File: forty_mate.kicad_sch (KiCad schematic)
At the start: 94 parts, among them SW1 SW_Push, SW10 SW_Push, SW11 SW_Push, SW12 SW_Push, SW13 SW_Push, SW14 SW_Push, SW15 SW_Push, SW16 SW_Push, SW17 SW_Push, SW18 SW_Push, SW19 SW_Push, SW2 SW_Push, SW20 SW_Push, SW21 SW_Push, SW22 SW_Push, SW23 SW_Push, SW24 SW_Push, SW25 SW_Push, SW26 SW_Push, SW27 SW_Push, SW28 SW_Push, SW29 SW_Push, SW3 SW_Push, SW30 SW_Push, SW31 SW_Push, SW32 SW_Push, SW33 SW_Push, SW34 SW_Push, SW35 SW_Push, SW36 SW_Push, SW37 SW_Push, SW38 SW_Push, SW39 SW_Push, SW4 SW_Push, SW40 SW_Push, SW41 SW_Push, SW42 SW_Push, SW43 SW_Push, SW44 SW_SPDT, SW5 SW_Push, SW6 SW_Push, SW7 SW_Push, SW8 SW_Push, SW9 SW_Push, U1 Micon_BLEMicroPro

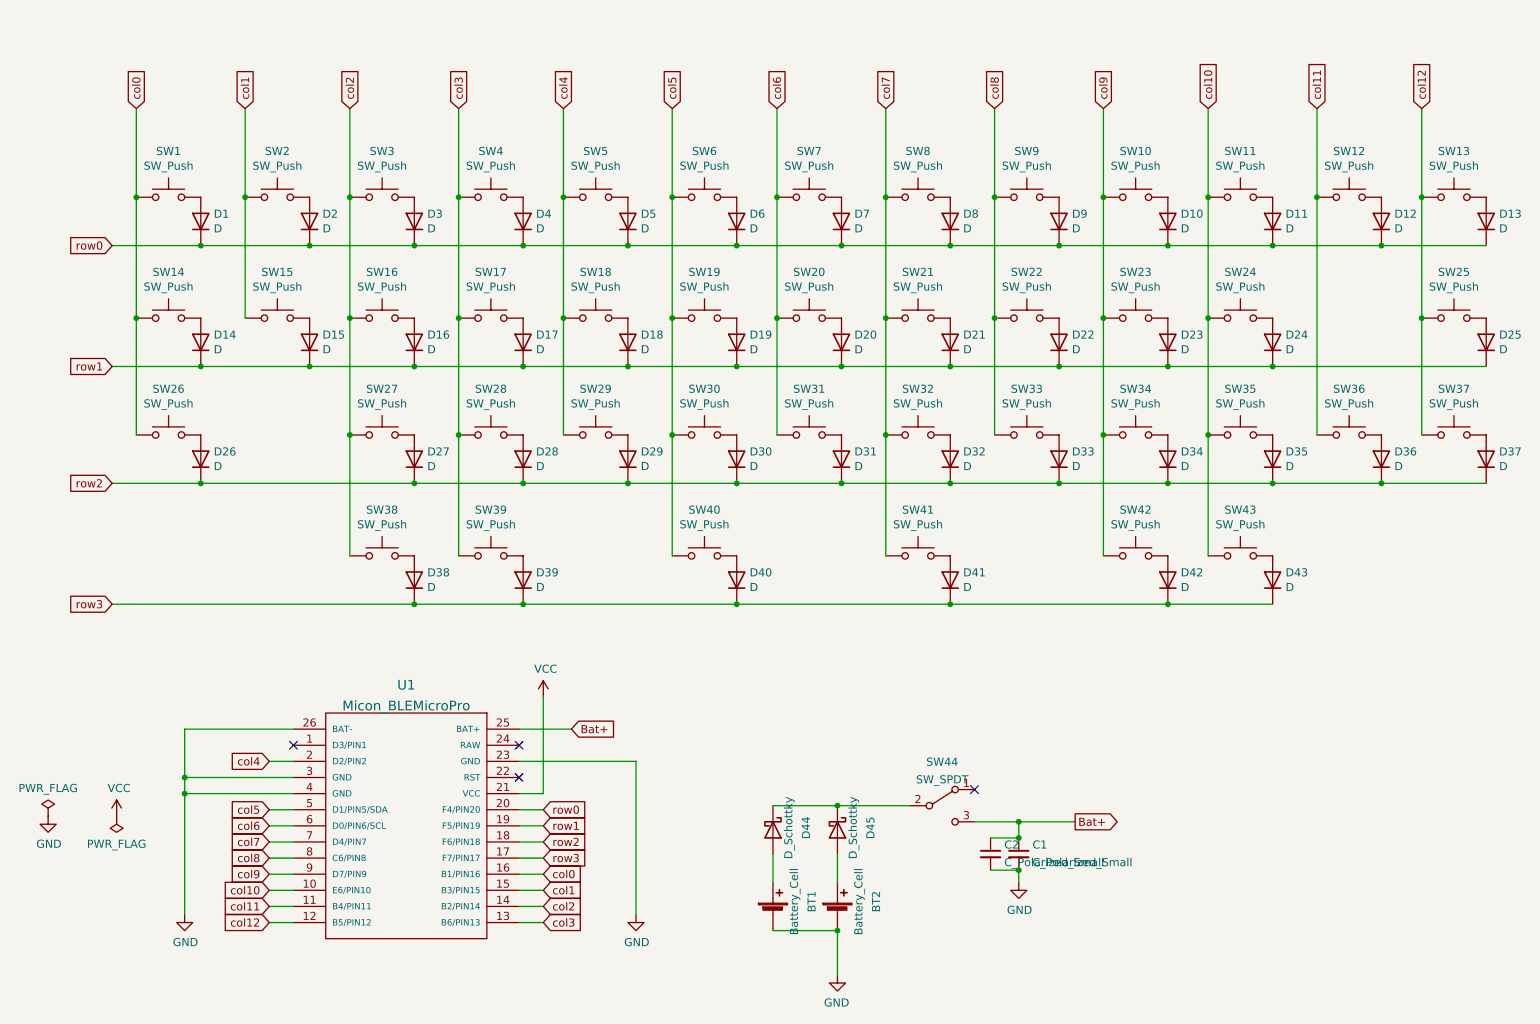
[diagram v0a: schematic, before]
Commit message: kari kansei
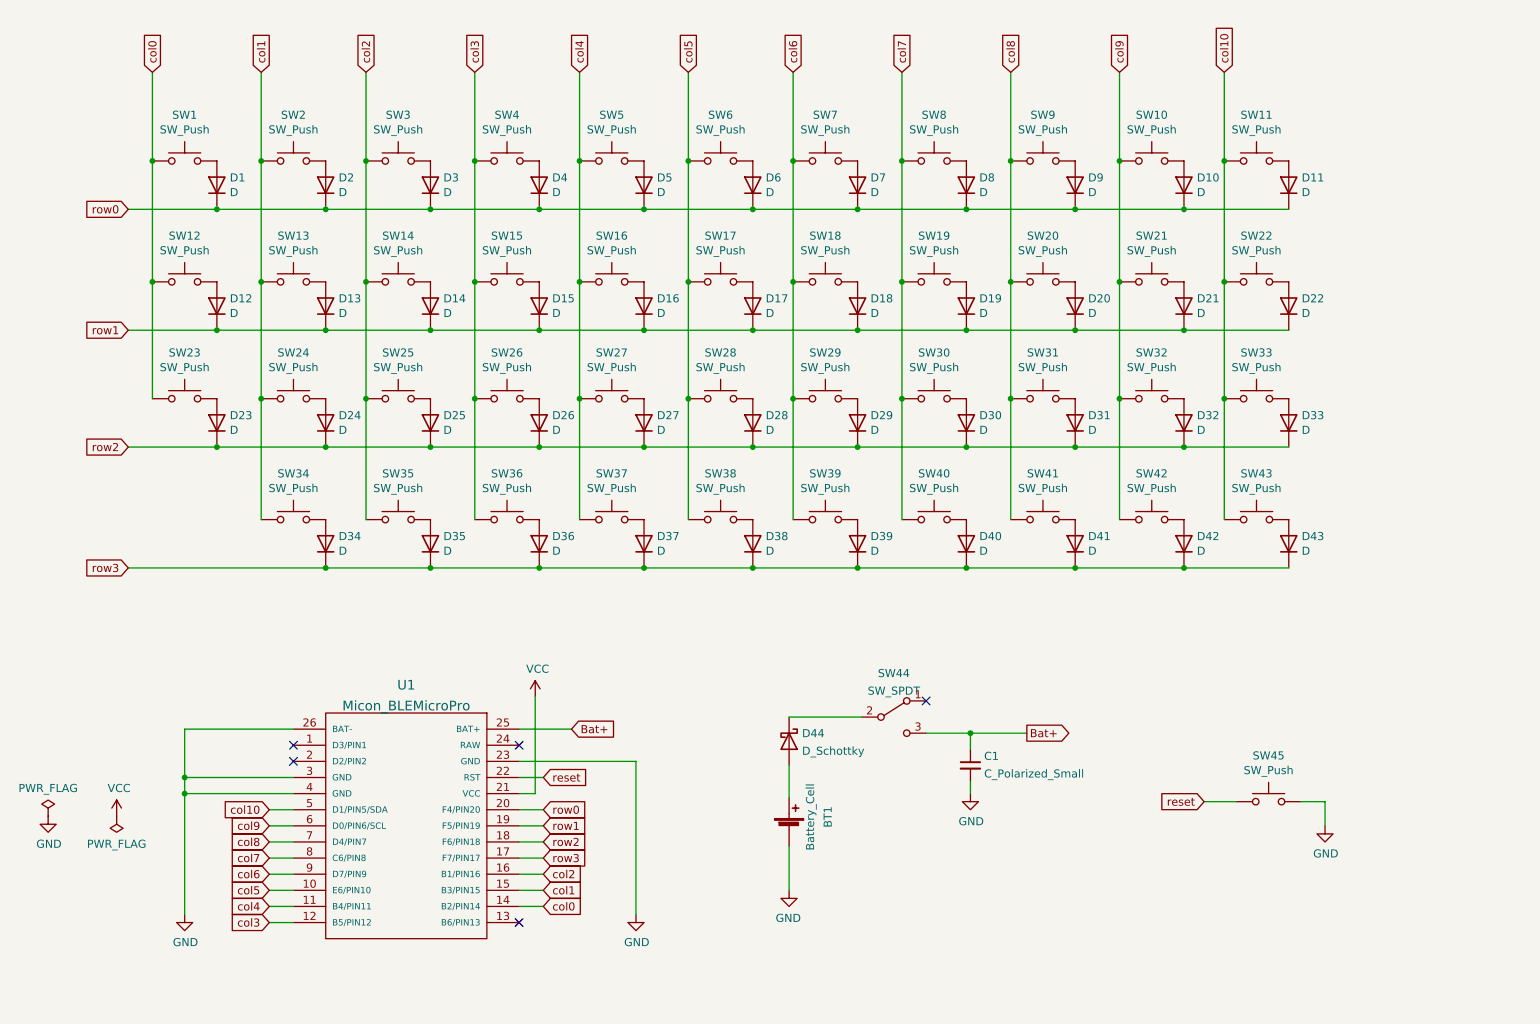
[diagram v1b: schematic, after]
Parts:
- removed BT1: Battery_Cell, kbd_Parts:Battery_ali_CR1632, symbol Device:Battery_Cell
- removed C2: C_Polarized_Small, kbd_Parts:Capacitor_1206, symbol Device:C_Small
- removed D12, D13, D25: D, kbd_Parts:Diode_TH_SMD, symbol Device:D
- removed D45: D_Schottky, kbd_Parts:Diode_TH_SMD, symbol Device:D_Schottky
- removed SW12, SW13, SW25: SW_Push, kbd_SW:CherryMX_Hotswap_1u, symbol Switch:SW_Push
- added D34, D39, D41: D, kbd_Parts:Diode_SMD, symbol Device:D
- added SW34, SW39, SW41: SW_Push, kbd_SW:CherryMX_Hotswap_1u, symbol Switch:SW_Push
- added SW45: SW_Push, kbd_Parts:ResetSW, symbol Switch:SW_Push
- D1, D10, D11, D2, D3, D37, D4, D42, D43, D5, D6, D7, D8, D9: footprint kbd_Parts:Diode_TH_SMD -> kbd_Parts:Diode_SMD
- D12: renamed from D14; footprint kbd_Parts:Diode_TH_SMD -> kbd_Parts:Diode_SMD
- D13: renamed from D15; footprint kbd_Parts:Diode_TH_SMD -> kbd_Parts:Diode_SMD
- D14: renamed from D16; footprint kbd_Parts:Diode_TH_SMD -> kbd_Parts:Diode_SMD
- D15: renamed from D17; footprint kbd_Parts:Diode_TH_SMD -> kbd_Parts:Diode_SMD
- D16: renamed from D18; footprint kbd_Parts:Diode_TH_SMD -> kbd_Parts:Diode_SMD
- D17: renamed from D19; footprint kbd_Parts:Diode_TH_SMD -> kbd_Parts:Diode_SMD
- D18: renamed from D20; footprint kbd_Parts:Diode_TH_SMD -> kbd_Parts:Diode_SMD
- D19: renamed from D21; footprint kbd_Parts:Diode_TH_SMD -> kbd_Parts:Diode_SMD
- D20: renamed from D22; footprint kbd_Parts:Diode_TH_SMD -> kbd_Parts:Diode_SMD
- D21: renamed from D23; footprint kbd_Parts:Diode_TH_SMD -> kbd_Parts:Diode_SMD
- D22: renamed from D24; footprint kbd_Parts:Diode_TH_SMD -> kbd_Parts:Diode_SMD
- D23: renamed from D26; footprint kbd_Parts:Diode_TH_SMD -> kbd_Parts:Diode_SMD
- D24: renamed from D36; footprint kbd_Parts:Diode_TH_SMD -> kbd_Parts:Diode_SMD
- D25: renamed from D27; footprint kbd_Parts:Diode_TH_SMD -> kbd_Parts:Diode_SMD
- D26: renamed from D28; footprint kbd_Parts:Diode_TH_SMD -> kbd_Parts:Diode_SMD
- D27: renamed from D29; footprint kbd_Parts:Diode_TH_SMD -> kbd_Parts:Diode_SMD
- D28: renamed from D30; footprint kbd_Parts:Diode_TH_SMD -> kbd_Parts:Diode_SMD
- D29: renamed from D31; footprint kbd_Parts:Diode_TH_SMD -> kbd_Parts:Diode_SMD
- D30: renamed from D32; footprint kbd_Parts:Diode_TH_SMD -> kbd_Parts:Diode_SMD
- D31: renamed from D33; footprint kbd_Parts:Diode_TH_SMD -> kbd_Parts:Diode_SMD
- D32: renamed from D34; footprint kbd_Parts:Diode_TH_SMD -> kbd_Parts:Diode_SMD
- D33: renamed from D35; footprint kbd_Parts:Diode_TH_SMD -> kbd_Parts:Diode_SMD
- D35: renamed from D38; footprint kbd_Parts:Diode_TH_SMD -> kbd_Parts:Diode_SMD
- D36: renamed from D39; footprint kbd_Parts:Diode_TH_SMD -> kbd_Parts:Diode_SMD
- D38: renamed from D40; footprint kbd_Parts:Diode_TH_SMD -> kbd_Parts:Diode_SMD
- D40: renamed from D41; footprint kbd_Parts:Diode_TH_SMD -> kbd_Parts:Diode_SMD
- D44: footprint kbd_Parts:Diode_TH_SMD -> forty_mate:Diode_SMD_S-FLAT
- SW12: renamed from SW14; footprint kbd_SW:CherryMX_Hotswap_1u -> kbd_SW:CherryMX_Hotswap_1.25u
- SW23: renamed from SW26; footprint kbd_SW:CherryMX_Hotswap_1u -> kbd_SW:CherryMX_Hotswap_1.75u
- SW35: renamed from SW38; footprint kbd_SW:CherryMX_Hotswap_1u -> kbd_SW:CherryMX_Hotswap_1.25u
- SW36: renamed from SW39; footprint kbd_SW:CherryMX_Hotswap_1u -> kbd_SW:CherryMX_Hotswap_2u_Rev
- SW37: footprint kbd_SW:CherryMX_Hotswap_1u -> kbd_SW:CherryMX_Hotswap_2.25u_Rev
- SW38: renamed from SW40; footprint kbd_SW:CherryMX_Hotswap_1u -> kbd_SW:CherryMX_Hotswap_1.25u
- SW42: footprint kbd_SW:CherryMX_Hotswap_1u -> kbd_SW:CherryMX_Hotswap_1.25u
- SW43: footprint kbd_SW:CherryMX_Hotswap_1u -> kbd_SW:CherryMX_Hotswap_1.75u
- renumbered BT2 to BT1, SW15 to SW13, SW16 to SW14, SW17 to SW15, SW18 to SW16, SW19 to SW17, SW20 to SW18, SW21 to SW19, SW22 to SW20, SW23 to SW21, SW24 to SW22, SW36 to SW24, SW27 to SW25, SW28 to SW26, SW29 to SW27, SW30 to SW28, SW31 to SW29, SW32 to SW30, SW33 to SW31, SW34 to SW32, SW35 to SW33, SW41 to SW40
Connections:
- net GND: now also SW45.2
- net col0: now also U1.14 (B2/PIN14); no longer U1.16 (B1/PIN16)
- net col1: now also SW24.1, SW34.1
- net col10: now also U1.5 (D1/PIN5/SDA); no longer U1.10 (E6/PIN10)
- net col2: now also U1.16 (B1/PIN16); no longer U1.14 (B2/PIN14)
- net col3: now also U1.12 (B5/PIN12); no longer U1.13 (B6/PIN13)
- net col4: now also SW37.1, U1.11 (B4/PIN11); no longer U1.2 (D2/PIN2)
- net col5: now also U1.10 (E6/PIN10); no longer U1.5 (D1/PIN5/SDA)
- net col6: now also U1.9 (D7/PIN9), SW39.1; no longer U1.6 (D0/PIN6/SCL)
- net col7: now also U1.8 (C6/PIN8); no longer U1.7 (D4/PIN7)
- net col8: now also U1.7 (D4/PIN7), SW41.1; no longer U1.8 (C6/PIN8)
- net col9: now also U1.6 (D0/PIN6/SCL); no longer U1.9 (D7/PIN9)
- net row2: no longer D37.1 (K)
- net row3: now also D37.1 (K), D34.1 (K), D39.1 (K), D41.1 (K)
- net at D44.2 (A): now also BT1.1 (+)
- net reset: now reaches U1.22 (RST)
- net reset: now also SW45.1
- removed net col11: SW24.1, U1.11 (B4/PIN11)
- removed net col12: SW37.1, U1.12 (B5/PIN12)
- new net: D34.2 (A), SW34.2
- new net: D39.2 (A), SW39.2
- new net: D41.2 (A), SW41.2
- no-connect marks 4 -> 5
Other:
- moved on the sheet: BT1, C1, D1, D10, D11, D12, D13, D14, D15, D16, D17, D18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

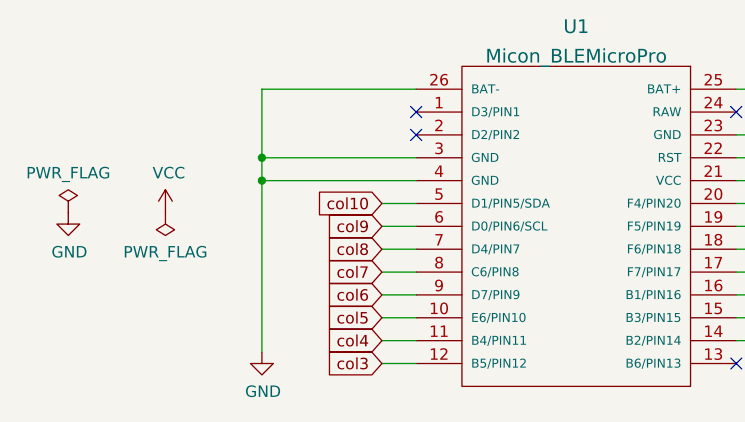
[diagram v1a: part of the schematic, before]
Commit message: add switch-plate and more change (true second proto) micon is inside out. changed cell box. switch no tokoro egutte mita
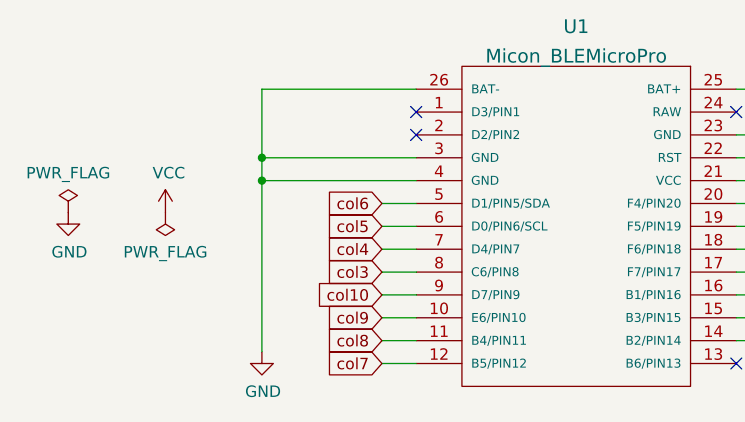
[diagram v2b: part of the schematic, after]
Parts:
- BT1: footprint kbd_Parts:Battery_ali_CR1632 -> forty_mate:HU1632
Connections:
- net col10: now also U1.9 (D7/PIN9); no longer U1.5 (D1/PIN5/SDA)
- net col3: now also U1.8 (C6/PIN8); no longer U1.12 (B5/PIN12)
- net col4: now also U1.7 (D4/PIN7); no longer U1.11 (B4/PIN11)
- net col5: now also U1.6 (D0/PIN6/SCL); no longer U1.10 (E6/PIN10)
- net col6: now also U1.5 (D1/PIN5/SDA); no longer U1.9 (D7/PIN9)
- net col7: now also U1.12 (B5/PIN12); no longer U1.8 (C6/PIN8)
- net col8: now also U1.11 (B4/PIN11); no longer U1.7 (D4/PIN7)
- net col9: now also U1.10 (E6/PIN10); no longer U1.6 (D0/PIN6/SCL)
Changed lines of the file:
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@@
     (stroke (width 0) (type default) (color 0 0 0 0))
   )
-  (global_label "col8" (shape input) (at 74.295 153.67 180) (fields_autoplaced)
+  (global_label "col8" (shape input) (at 74.295 163.83 180) (fields_autoplaced)
     (effects (font (size 1.27 1.27)) (justify right))
-    (property "シート間のリファレンス" "${INTERSHEET_REFS}" (id 0) (at 161.29 203.2 0)
+    (property "シート間のリファレンス" "${INTERSHEET_REFS}" (id 0) (at 161.29 213.36 0)
       (effects (font (size 1.27 1.27)) hide)
     )
@@
     )
   )
-  (global_label "col4" (shape input) (at 74.295 163.83 180) (fields_autoplaced)
+  (global_label "col4" (shape input) (at 74.295 153.67 180) (fields_autoplaced)
     (effects (font (size 1.27 1.27)) (justify right))
-    (property "シート間のリファレンス" "${INTERSHEET_REFS}" (id 0) (at 15.24 104.14 0)
+    (property "シート間のリファレンス" "${INTERSHEET_REFS}" (id 0) (at 15.24 93.98 0)
       (effects (font (size 1.27 1.27)) hide)
     )
@@
     )
   )
-  (global_label "col7" (shape input) (at 74.295 156.21 180) (fields_autoplaced)
+  (global_label "col7" (shape input) (at 74.295 166.37 180) (fields_autoplaced)
     (effects (font (size 1.27 1.27)) (justify right))
-    (property "シート間のリファレンス" "${INTERSHEET_REFS}" (id 0) (at 161.29 203.2 0)
-      (effects (font (size 1.27 1.27)) hide)
-    )
-  )
-  (global_label "col9" (shape input) (at 74.295 151.13 180) (fields_autoplaced)
+    (property "シート間のリファレンス" "${INTERSHEET_REFS}" (id 0) (at 161.29 213.36 0)
+      (effects (font (size 1.27 1.27)) hide)
+    )
+  )
+  (global_label "col9" (shape input) (at 74.295 161.29 180) (fields_autoplaced)
     (effects (font (size 1.27 1.27)) (justify right))
-    (property "シート間のリファレンス" "${INTERSHEET_REFS}" (id 0) (at 161.29 203.2 0)
+    (property "シート間のリファレンス" "${INTERSHEET_REFS}" (id 0) (at 161.29 213.36 0)
       (effects (font (size 1.27 1.27)) hide)
     )
@@
     )
   )
-  (global_label "col6" (shape input) (at 74.295 158.75 180) (fields_autoplaced)
+  (global_label "col6" (shape input) (at 74.295 148.59 180) (fields_autoplaced)
     (effects (font (size 1.27 1.27)) (justify right))
-    (property "シート間のリファレンス" "${INTERSHEET_REFS}" (id 0) (at 161.29 203.2 0)
+    (property "シート間のリファレンス" "${INTERSHEET_REFS}" (id 0) (at 161.29 193.04 0)
       (effects (font (size 1.27 1.27)) hide)
     )
@@
     )
   )
-  (global_label "col5" (shape input) (at 74.295 161.29 180) (fields_autoplaced)
+  (global_label "col5" (shape input) (at 74.295 151.13 180) (fields_autoplaced)
     (effects (font (size 1.27 1.27)) (justify right))
-    (property "シート間のリファレンス" "${INTERSHEET_REFS}" (id 0) (at 161.29 203.2 0)
+    (property "シート間のリファレンス" "${INTERSHEET_REFS}" (id 0) (at 161.29 193.04 0)
       (effects (font (size 1.27 1.27)) hide)
     )
@@
     )
   )
-  (global_label "col10" (shape input) (at 74.295 148.59 180) (fields_autoplaced)
+  (global_label "col10" (shape input) (at 74.295 158.75 180) (fields_autoplaced)
     (effects (font (size 1.27 1.27)) (justify right))
-    (property "シート間のリファレンス" "${INTERSHEET_REFS}" (id 0) (at 161.29 203.2 0)
-      (effects (font (size 1.27 1.27)) hide)
-    )
-  )
-  (global_label "col3" (shape input) (at 74.295 166.37 180) (fields_autoplaced)
+    (property "シート間のリファレンス" "${INTERSHEET_REFS}" (id 0) (at 161.29 213.36 0)
+      (effects (font (size 1.27 1.27)) hide)
+    )
+  )
+  (global_label "col3" (shape input) (at 74.295 156.21 180) (fields_autoplaced)
     (effects (font (size 1.27 1.27)) (justify right))
-    (property "シート間のリファレンス" "${INTERSHEET_REFS}" (id 0) (at 15.24 109.22 0)
+    (property "シート間のリファレンス" "${INTERSHEET_REFS}" (id 0) (at 15.24 99.06 0)
       (effects (font (size 1.27 1.27)) hide)
     )
@@
     (property "Reference" "BT1" (id 0) (at 162.3355 149.733 90))
     (property "Value" "Battery_Cell" (id 1) (at 159.5604 149.733 90))
-    (property "Footprint" "kbd_Parts:Battery_ali_CR1632" (id 2) (at 156.21 150.241 90)
+    (property "Footprint" "forty_mate:HU1632" (id 2) (at 156.21 150.241 90)
       (effects (font (size 1.27 1.27)) hide)
     )
@@
     )
     (path "/6d29fe29-40ca-41b0-a6c4-7f62498671f3"
-      (reference "BT1") (unit 1) (value "Battery_Cell") (footprint "kbd_Parts:Battery_ali_CR1632")
+      (reference "BT1") (unit 1) (value "Battery_Cell") (footprint "forty_mate:HU1632")
     )
     (path "/bd884d10-8c4b-40e4-90f1-6eb220af54c8"
